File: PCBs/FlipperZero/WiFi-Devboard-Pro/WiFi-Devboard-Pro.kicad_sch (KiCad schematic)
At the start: 35 parts, among them IC1 ESP32-WROOM-32E-N4, IC2 DMP1045U-7, IC3 AZ1117H-3.3TRE1, IC4 DMP1045U-7, IC5 DMP1045U-7, J1 3220-10-0300-00, J2 X6511WVS-08H-C60D48R2, J3 DZ254S-11-10-48, J4 Conn_01x11, J5 Conn_01x11, J6 503398-1892, U1 MMDT2907A-7-F, U2 MMDT2907A-7-F, U3 MMDT2907A-7-F

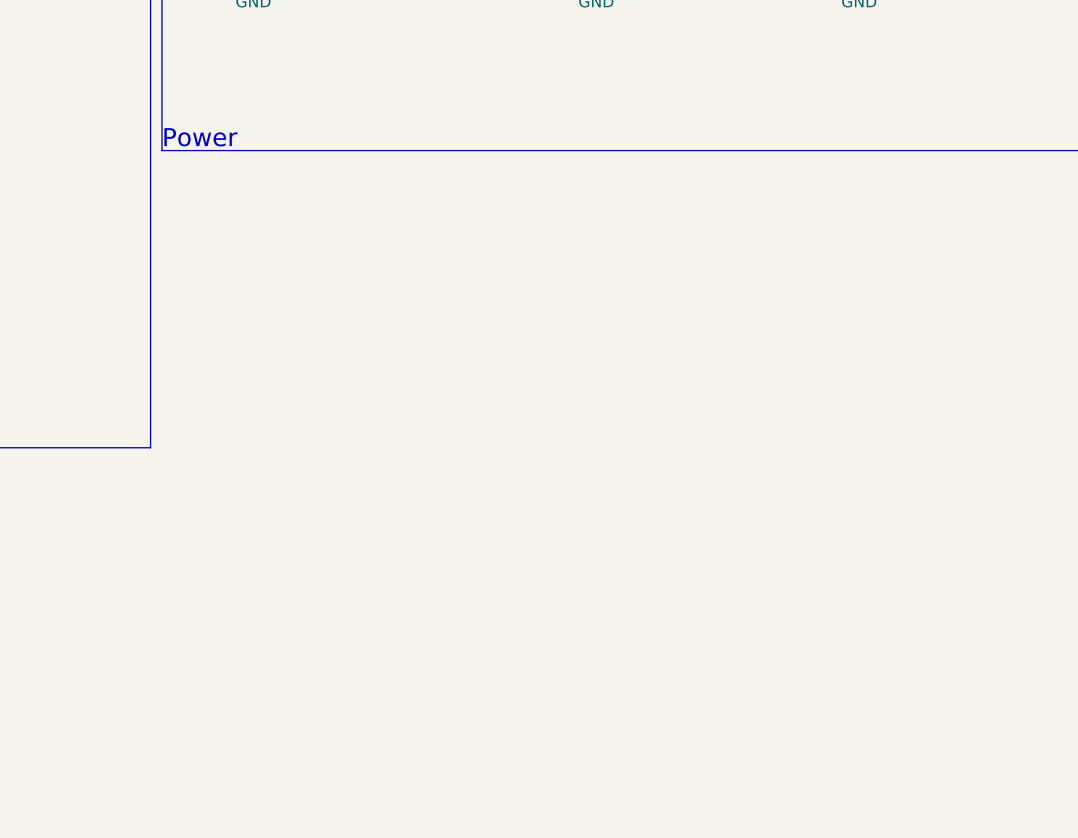
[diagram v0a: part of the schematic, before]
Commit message: Place components on PCB
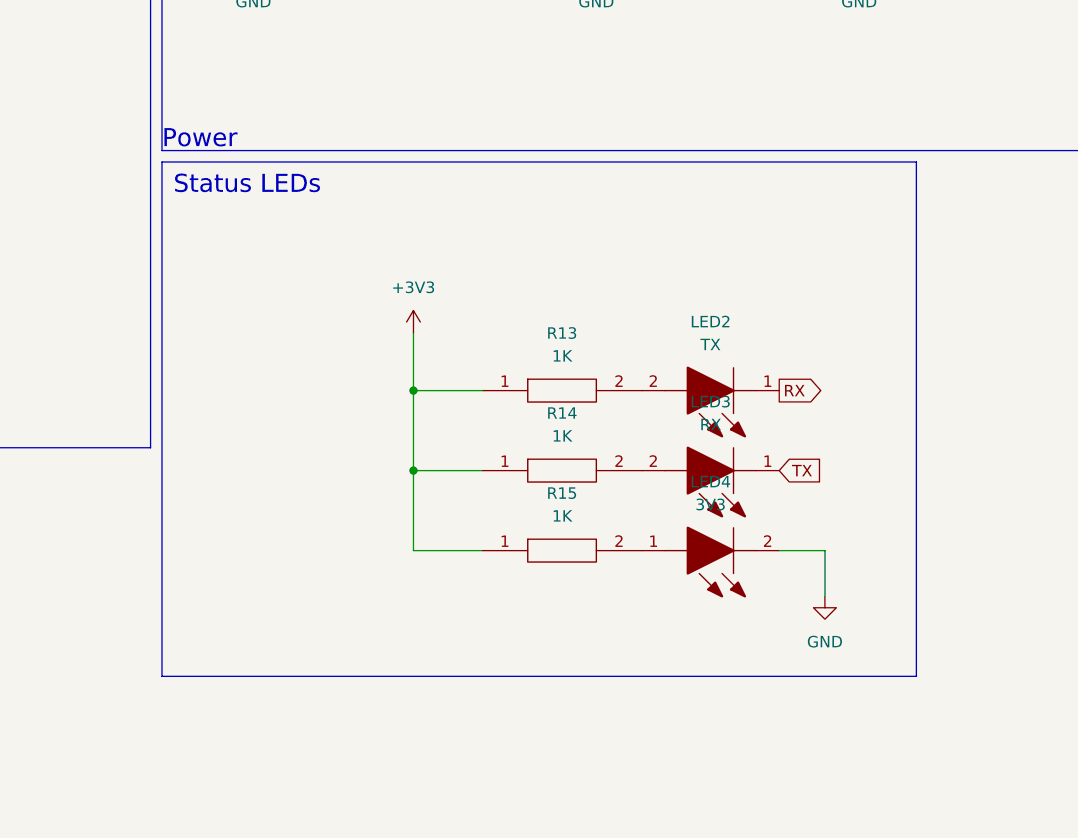
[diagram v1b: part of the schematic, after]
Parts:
- added LED2: TX, LEDC1608X50N, symbol SamacSys_Parts:19-217_Y5C-AP1Q2_3T
- added LED3: RX, LEDC1608X50N, symbol SamacSys_Parts:19-217_Y5C-AP1Q2_3T
- added LED4: 3V3, 19217R6CAL1M2VY3T, symbol SamacSys_Parts:19-217_R6C-AL1M2VY_3T
- added R13, R14, R15: 1K, RESC1005X40N, symbol SamacSys_Parts:RC0402FR-071KL
- J4, J5: footprint (none) -> Connector_PinHeader_2.54mm:PinHeader_1x11_P2.54mm_Vertical
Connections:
- net +3V3: now also R13.1, R14.1, R15.1
- net GND: now also LED4.2
- net RX: now also LED2.1
- net TX: now also LED3.1
- new net: LED3.2, R14.2
- new net: LED2.2, R13.2
- new net: LED4.1, R15.2
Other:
- note added: "Status LEDs"
